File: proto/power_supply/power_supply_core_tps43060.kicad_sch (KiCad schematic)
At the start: 46 parts, among them Q202 TK4R3E06PL, Q203 TK4R3E06PL, U101 ZXCT1110, U203 TPS43060

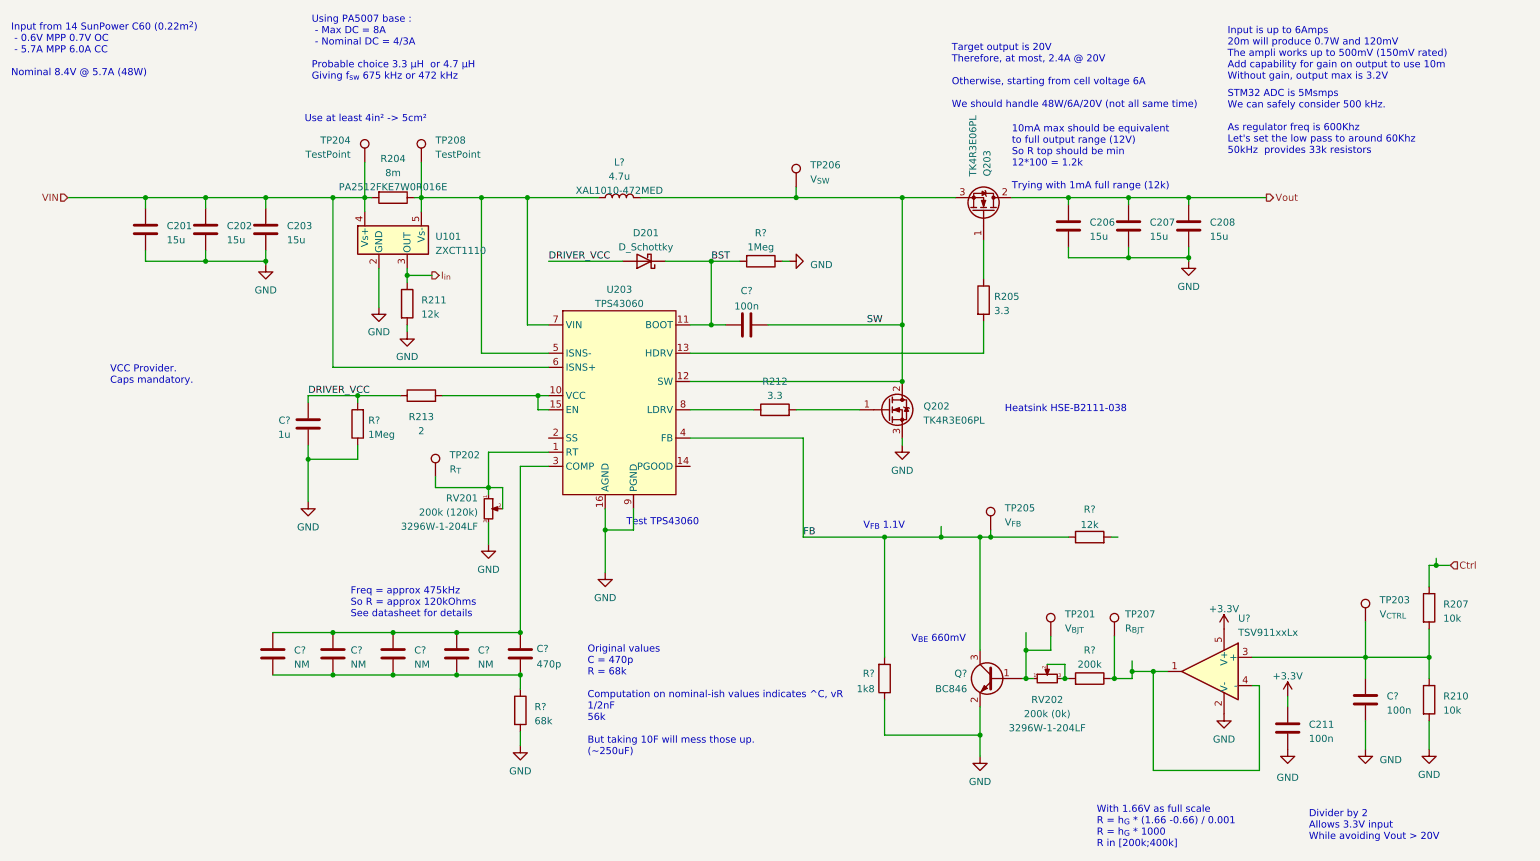
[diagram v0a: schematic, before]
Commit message: Finish alim sch, start PCB
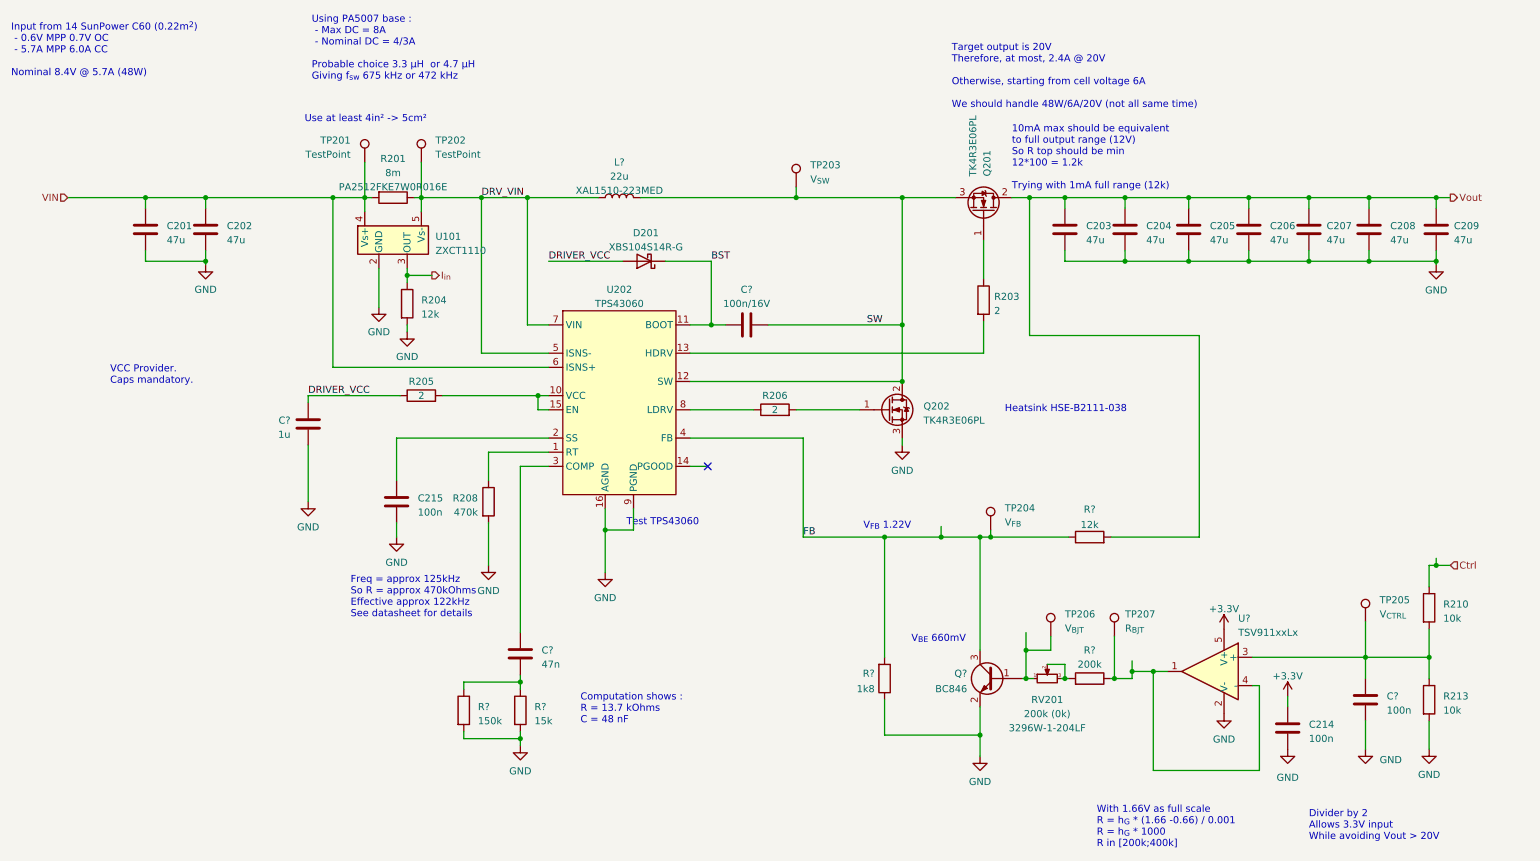
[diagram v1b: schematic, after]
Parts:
- removed C? (x4): NM, Capacitor_SMD:C_0805_2012Metric, symbol Device:C
- removed R? (x2): 1Meg, Resistor_SMD:R_0805_2012Metric, symbol Device:R
- removed RV201: 200k (120k), Potentiometer_THT:Potentiometer_Bourns_3296W_Vertical, symbol Device:R_Potentiometer_Small
- removed TP202: R_{T}, TestPoint:TestPoint_Keystone_5010-5014_Multipurpose, symbol Connector:TestPoint
- added C204, C208, C209: 47u, Capacitor_SMD:C_1206_3216Metric, symbol Device:C
- added C215: 100n, Capacitor_SMD:C_0805_2012Metric, symbol Device:C
- added R208: 470k, Resistor_SMD:R_0805_2012Metric, symbol Device:R
- added R?: 150k, Resistor_SMD:R_0805_2012Metric, symbol Device:R
- C201, C202, C203: value 15u -> 47u; footprint Capacitor_SMD:C_0805_2012Metric -> Capacitor_SMD:C_1206_3216Metric
- C205: renamed from C206; value 15u -> 47u; footprint Capacitor_SMD:C_0805_2012Metric -> Capacitor_SMD:C_1206_3216Metric
- C206: renamed from C207; value 15u -> 47u; footprint Capacitor_SMD:C_0805_2012Metric -> Capacitor_SMD:C_1206_3216Metric
- C207: renamed from C208; value 15u -> 47u; footprint Capacitor_SMD:C_0805_2012Metric -> Capacitor_SMD:C_1206_3216Metric
- C?: value 470p -> 47n
- C?: value 100n -> 100n/16V
- D201: value D_Schottky -> XBS104S14R-G; footprint (none) -> Diode_SMD:D_SOD-123
- L?: value 4.7u -> 22u; footprint Inductor_SMD:L_Coilcraft_XAL1010-XXX -> Inductor_SMD:L_Coilcraft_XAL1510-223; MPN XAL1010-472MED -> XAL1510-223MED
- R203: renamed from R205; value 3.3 -> 2; footprint (none) -> Resistor_SMD:R_0805_2012Metric
- R205: renamed from R213; footprint (none) -> Resistor_SMD:R_0805_2012Metric
- R206: renamed from R212; value 3.3 -> 2; footprint (none) -> Resistor_SMD:R_0805_2012Metric
- R?: value 68k -> 15k
- renumbered C211 to C214, Q203 to Q201, R204 to R201, R211 to R204, R207 to R210, R210 to R213, RV202 to RV201, TP204 to TP201, TP208 to TP202, TP206 to TP203, TP205 to TP204, TP203 to TP205, TP201 to TP206, U203 to U202
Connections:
- net GND: now also C204.2, C208.2, C209.2, C215.2, R208.2, R?.2
- net VIN: no longer C203.1
- net Vout: now also C203.1, R?.2, C204.1, C208.1, C209.1
- net DRV_VIN: now reaches L?.1, R201.1, TP202.1, U101.5 (Vs-), U202.5 (ISNS-), U202.7 (VIN)
- net at U202.1 (RT): now also R208.1
- net at C?.2, R?.1: now also R?.1
- net at U202.2 (SS): now also C215.1
- no-connect marks 0 -> 1
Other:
- note added: "Computation shows : R = 13.7 kOhms C = 48 nF"
- note added: "Freq = approx 125kHz So R = approx 470kOhms Effective approx 122kHz See datasheet for details"
- note added: "V_{FB} 1.22V"
- note removed: "Freq = approx 475kHz So R = approx 120kOhms See datasheet for details"
- note removed: "Input is up to 6Amps 20m will produce 0.7W and 120mV The ampli works up to 500mV (150mV rated) Add capability for gain on output to use 10m Without gain, output max is 3.2V"
- note removed: "Original values C = 470p R = 68k Computation on nominal-ish values indicates ^C, vR 1/2nF 56k But taking 10F will mess those up. (~250uF)"
- note removed: "STM32 ADC is 5Msmps We can safely consider 500 kHz. As regulator freq is 600Khz Let's set the low pass to around 60Khz 50kHz provides 33k resistors"
- note removed: "V_{FB} 1.1V"
- moved on the sheet: C205, C206, C207
